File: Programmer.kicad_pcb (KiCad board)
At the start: 2 copper layers, 76.2 x 50.8 mm, 78 parts, among them CON1 USB_OTG, M1 ESP-12E, P1 CONN_01X12, P3 CONN_12, Q1 BSS138L, Q2 MMBT3906, Q3 MMBT3904, Q4 BSS84, Q5 BSS138L, Q7 MMBT3904, Q8 MMBT3904, SW1 RESET, U1 AP2112K-3.3, U10 NC7SB3157, U2 23LC1024, U3 TXS0108PWR, U4 AAT3672-4.2-1, U8 CH340G, Y1 12 Mhz

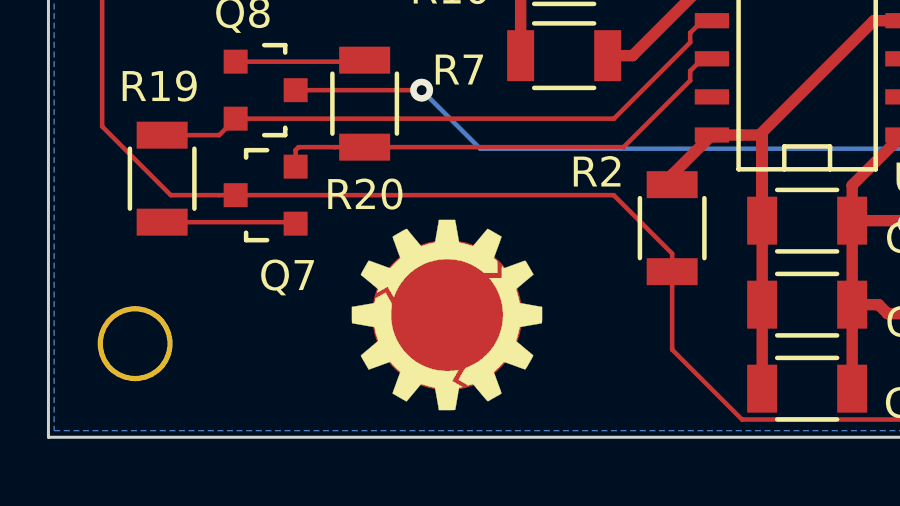
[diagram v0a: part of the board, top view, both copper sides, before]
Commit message: Minor Changes
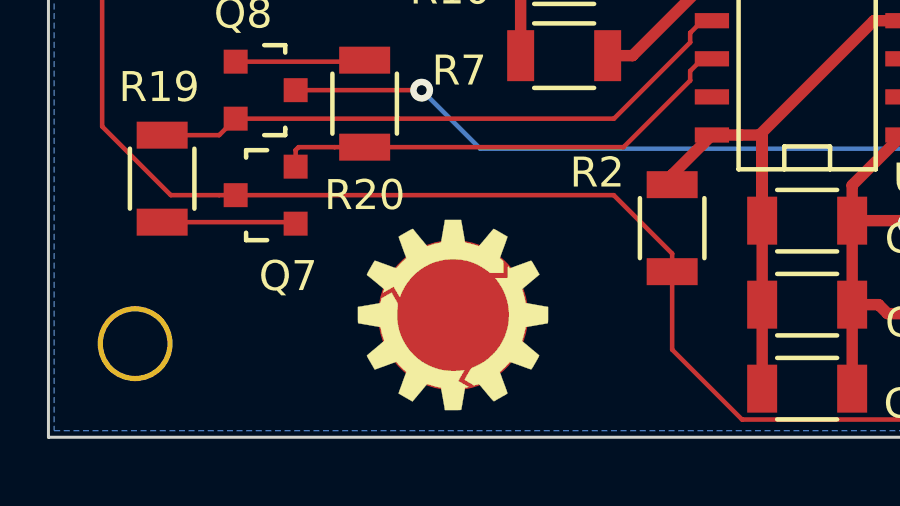
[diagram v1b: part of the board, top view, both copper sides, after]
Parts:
- moved Ref** 0.20 mm to (64.3, 83.0)
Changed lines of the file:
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@@
     (links 0)
     (no_connects 0)
-    (area 50.759999 36.269999 127.060001 87.170001)
+    (area 43.573791 30.539016 146.5274 107.0334)
     (thickness 1.6)
     (drawings 7)
@@
     (visible_elements FFFFEF7F)
     (pcbplotparams
-      (layerselection 0x0103c_80000001)
+      (layerselection 0x010e0_80000001)
       (usegerberextensions false)
       (excludeedgelayer true)
@@
   )
   (module UprogrammerFPs:PILogo1 (layer F.Cu)
-    (at 64.1 83.05)
+    (at 64.3 83.05)
     (fp_text reference Ref** (at -1.5 -4) (layer F.Fab) hide
       (effects (font (thickness 0.15)))
